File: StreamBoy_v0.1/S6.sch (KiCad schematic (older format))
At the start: 27 parts, among them U1 XC6SLX9-TQG144

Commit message: I hate component placement!
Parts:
- R20, R21, R22, R5, R8: footprint Resistor_SMD:R_0805_2012Metric -> Resistor_SMD:R_0402_1005Metric; lcscPartnum (none) -> C25900
- R6: footprint Resistor_SMD:R_0805_2012Metric -> Resistor_SMD:R_0402_1005Metric; lcscPartnum (none) -> C25890
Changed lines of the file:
@@
 F 0 "R5" V 7070 9746 50  0000 L CNN
 F 1 "4.7KOhm" V 7150 9550 50  0000 L CNN
-F 2 "Resistor_SMD:R_0805_2012Metric" V 6930 9700 50  0001 C CNN
+F 2 "Resistor_SMD:R_0402_1005Metric" V 6930 9700 50  0001 C CNN
 F 3 "~" H 7000 9700 50  0001 C CNN
+F 4 "C25900" H 7000 9700 50  0001 C CNN "lcscPartnum"
 	1    7000 9700
 	0    -1   -1   0
@@
 F 0 "R8" V 5270 8646 50  0000 L CNN
 F 1 "4.7KOhm" V 5350 8450 50  0000 L CNN
-F 2 "Resistor_SMD:R_0805_2012Metric" V 5130 8600 50  0001 C CNN
+F 2 "Resistor_SMD:R_0402_1005Metric" V 5130 8600 50  0001 C CNN
 F 3 "~" H 5200 8600 50  0001 C CNN
+F 4 "C25900" H 5200 8600 50  0001 C CNN "lcscPartnum"
 	1    5200 8600
 	0    1    1    0
@@
 F 0 "R20" V 7070 9396 50  0000 L CNN
 F 1 "4.7KOhm" V 7150 9200 50  0000 L CNN
-F 2 "Resistor_SMD:R_0805_2012Metric" V 6930 9350 50  0001 C CNN
+F 2 "Resistor_SMD:R_0402_1005Metric" V 6930 9350 50  0001 C CNN
 F 3 "~" H 7000 9350 50  0001 C CNN
+F 4 "C25900" H 7000 9350 50  0001 C CNN "lcscPartnum"
 	1    7000 9350
 	0    -1   -1   0
@@
 F 0 "R6" V 7070 9046 50  0000 L CNN
 F 1 "330Ohm" V 7150 8850 50  0000 L CNN
-F 2 "Resistor_SMD:R_0805_2012Metric" V 6930 9000 50  0001 C CNN
+F 2 "Resistor_SMD:R_0402_1005Metric" V 6930 9000 50  0001 C CNN
 F 3 "~" H 7000 9000 50  0001 C CNN
+F 4 "C25890" H 7000 9000 50  0001 C CNN "lcscPartnum"
 	1    7000 9000
 	0    -1   -1   0
@@
 F 0 "R21" V 7070 10096 50  0000 L CNN
 F 1 "4.7KOhm" V 7150 9900 50  0000 L CNN
-F 2 "Resistor_SMD:R_0805_2012Metric" V 6930 10050 50  0001 C CNN
+F 2 "Resistor_SMD:R_0402_1005Metric" V 6930 10050 50  0001 C CNN
 F 3 "~" H 7000 10050 50  0001 C CNN
+F 4 "C25900" H 7000 10050 50  0001 C CNN "lcscPartnum"
 	1    7000 10050
 	0    -1   -1   0
@@
 F 0 "R22" V 7070 10446 50  0000 L CNN
 F 1 "4.7KOhm" V 7150 10250 50  0000 L CNN
-F 2 "Resistor_SMD:R_0805_2012Metric" V 6930 10400 50  0001 C CNN
+F 2 "Resistor_SMD:R_0402_1005Metric" V 6930 10400 50  0001 C CNN
 F 3 "~" H 7000 10400 50  0001 C CNN
+F 4 "C25900" H 7000 10400 50  0001 C CNN "lcscPartnum"
 	1    7000 10400
 	0    -1   -1   0

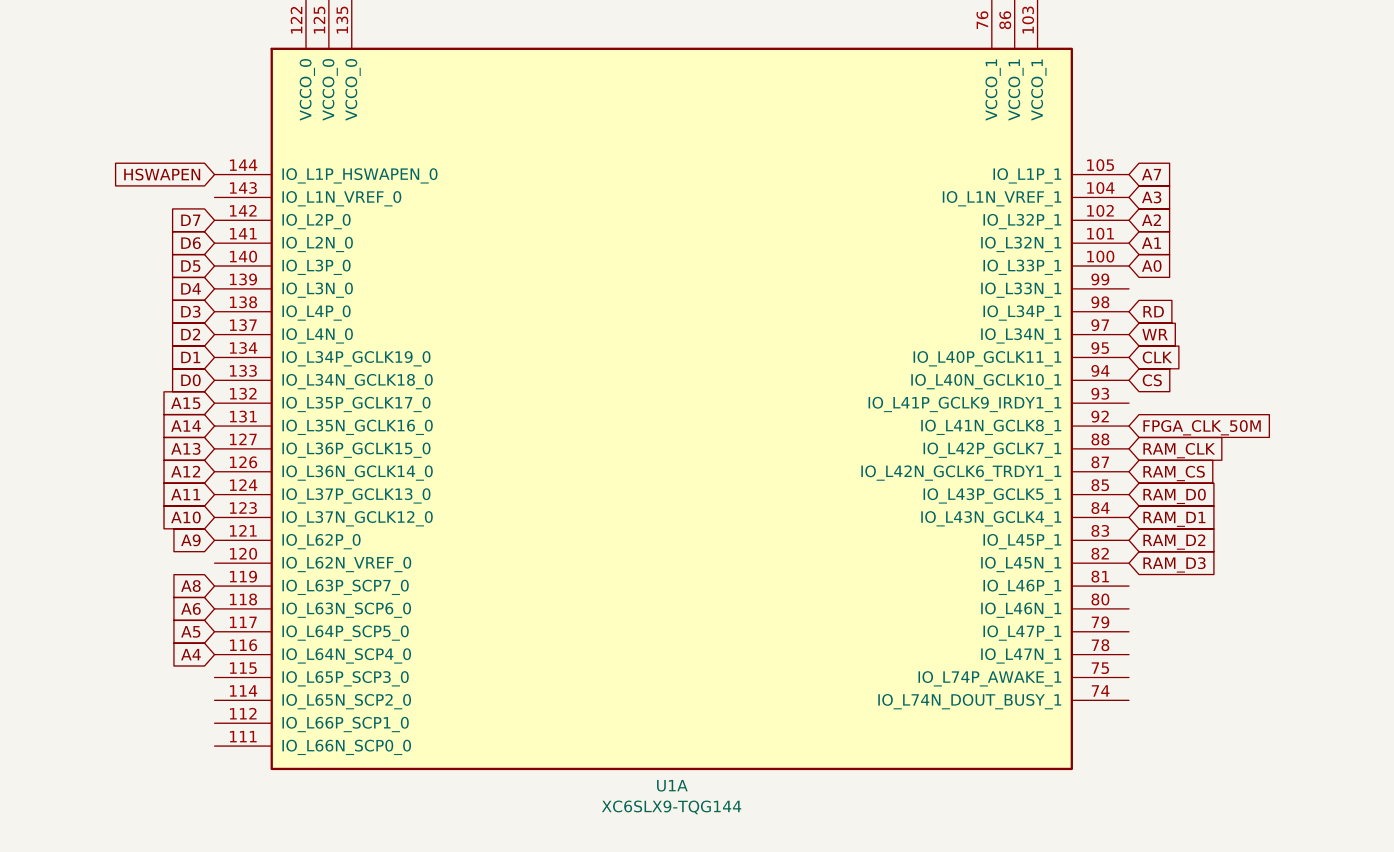
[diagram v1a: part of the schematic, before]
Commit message: Started to route some stuff
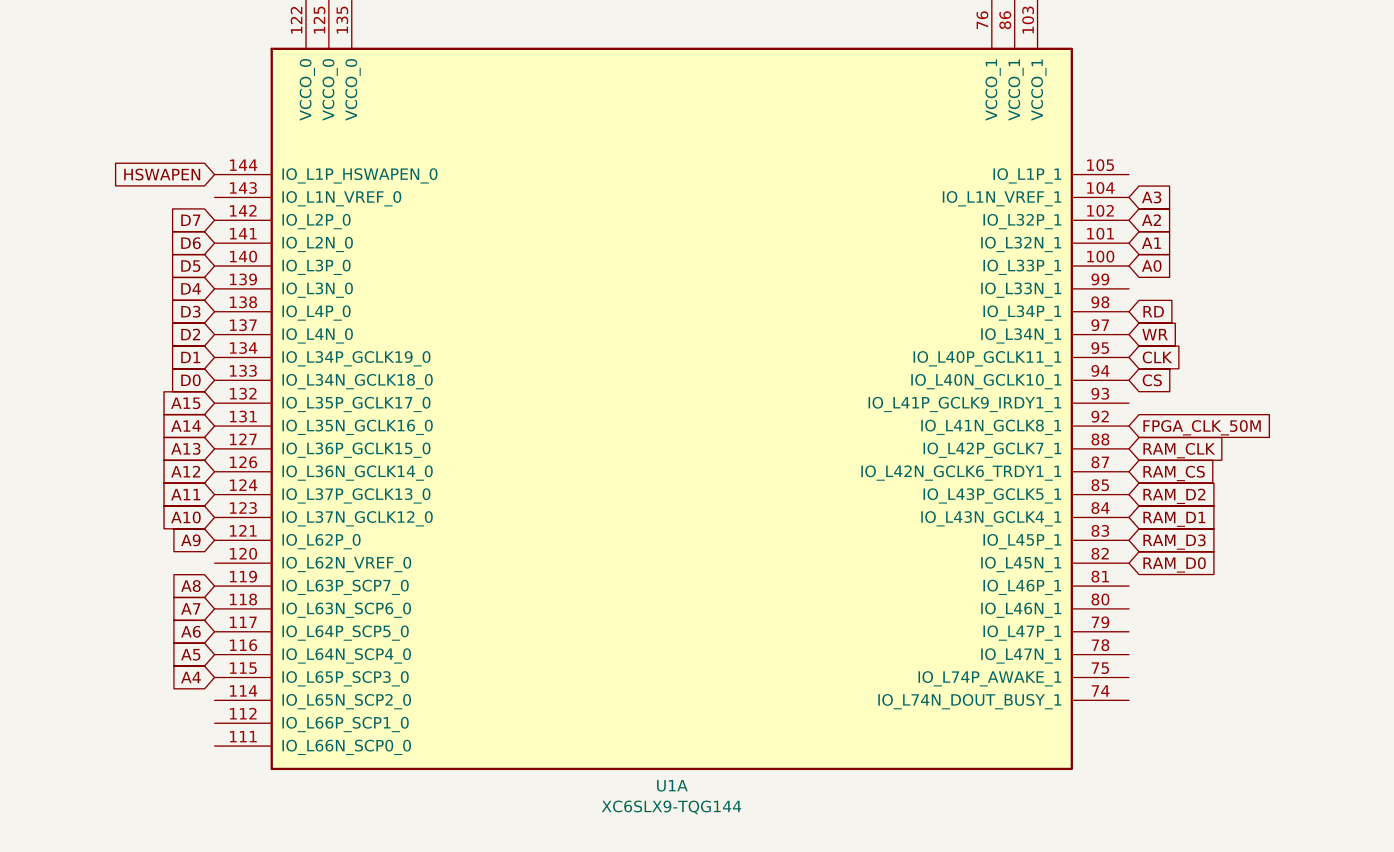
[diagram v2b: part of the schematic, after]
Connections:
- net A4: now also U1.115 (IO_L65P_SCP3_0); no longer U1.116 (IO_L64N_SCP4_0)
- net A5: now also U1.116 (IO_L64N_SCP4_0); no longer U1.117 (IO_L64P_SCP5_0)
- net A6: now also U1.117 (IO_L64P_SCP5_0); no longer U1.118 (IO_L63N_SCP6_0)
- net A7: now also U1.118 (IO_L63N_SCP6_0); no longer U1.105 (IO_L1P_1)
- net RAM_D0: now also U1.82 (IO_L45N_1); no longer U1.85 (IO_L43P_GCLK5_1)
- net RAM_D2: now also U1.85 (IO_L43P_GCLK5_1); no longer U1.83 (IO_L45P_1)
- net RAM_D3: now also U1.83 (IO_L45P_1); no longer U1.82 (IO_L45N_1)
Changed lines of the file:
@@
 Text GLabel 6450 3150 2    50   Input ~ 0
 RAM_CS
-Text GLabel 6450 3250 2    50   Input ~ 0
+Text GLabel 6450 3550 2    50   Input ~ 0
 RAM_D0
 Text GLabel 6450 3350 2    50   Input ~ 0
 RAM_D1
+Text GLabel 6450 3250 2    50   Input ~ 0
+RAM_D2
 Text GLabel 6450 3450 2    50   Input ~ 0
-RAM_D2
-Text GLabel 6450 3550 2    50   Input ~ 0
 RAM_D3
 Text GLabel 13700 1950 2    50   Input ~ 0
@@
 Text GLabel 13700 2050 2    50   Input ~ 0
 FPGA_LED2
+Text GLabel 2450 4050 0    50   Input ~ 0
+A4
 Text GLabel 2450 3950 0    50   Input ~ 0
-A4
+A5
 Text GLabel 2450 3850 0    50   Input ~ 0
-A5
-Text GLabel 2450 3750 0    50   Input ~ 0
 A6
 Text GLabel 2450 3650 0    50   Input ~ 0
@@
 Text Notes 13850 1850 0    50   ~ 0
 Place anywhere
-Text GLabel 6450 1850 2    50   Input ~ 0
+Text GLabel 2450 3750 0    50   Input ~ 0
 A7
 Text GLabel 6450 1950 2    50   Input ~ 0
